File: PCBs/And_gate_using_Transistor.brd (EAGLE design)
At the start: 30 x 34.5 mm, 11 parts, among them T1 BC547, T2 BC547

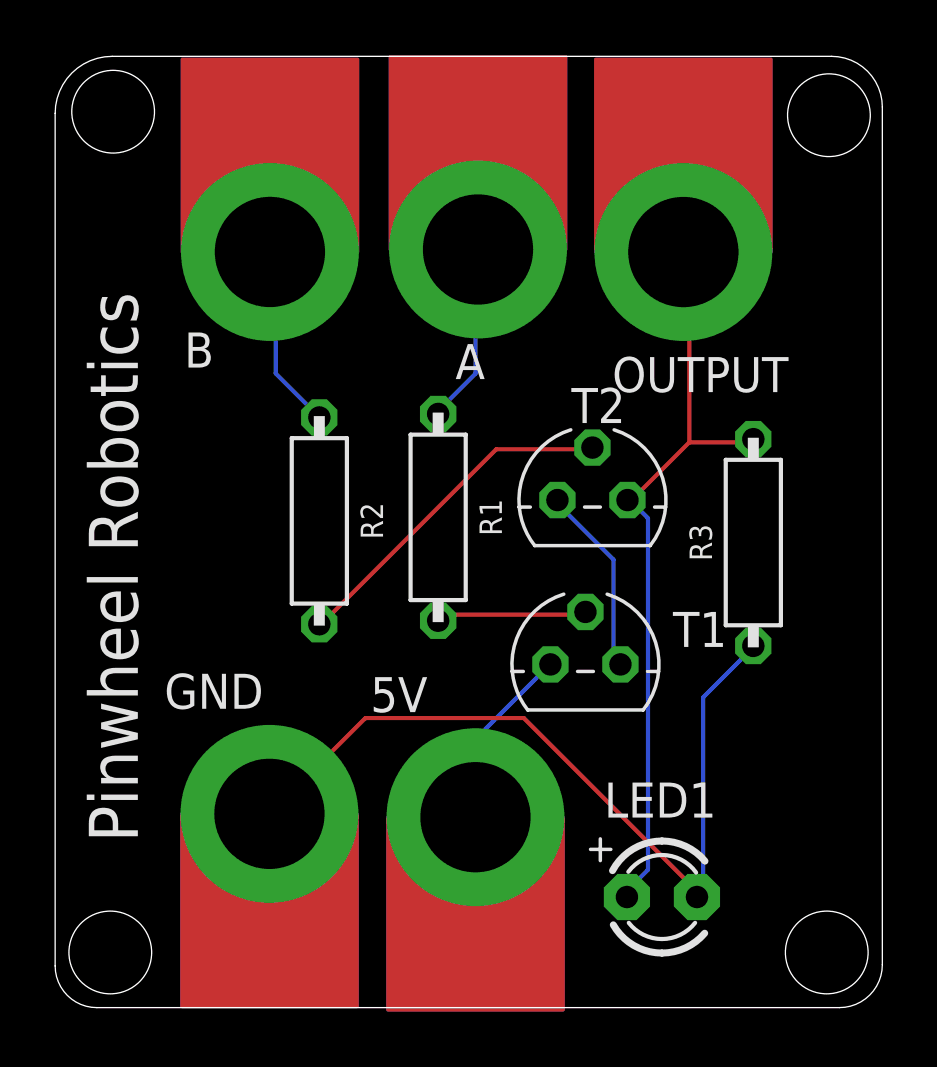
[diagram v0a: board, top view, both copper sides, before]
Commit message: New Update
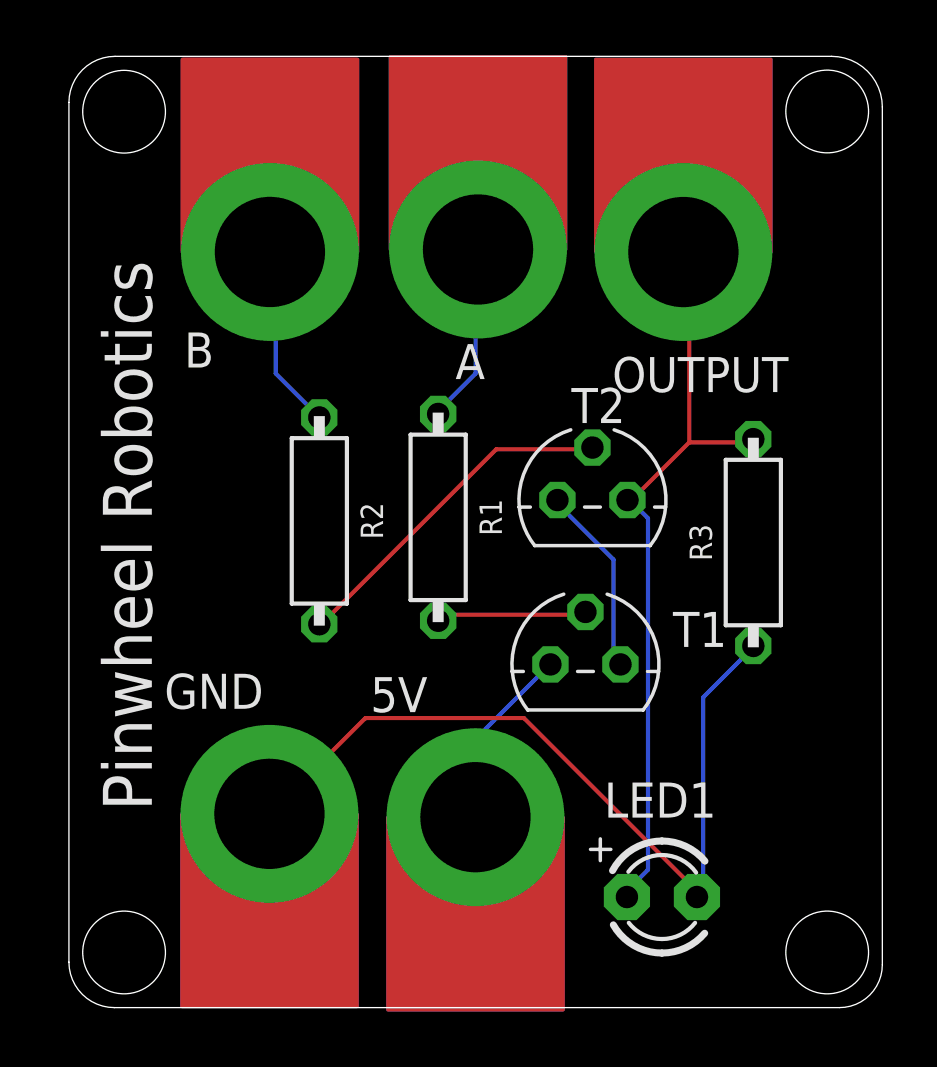
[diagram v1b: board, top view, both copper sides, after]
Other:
- board size 30 x 34.5 mm -> 29.5 x 34.5 mm
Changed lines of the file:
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@@
 <drawing>
 <settings>
-<setting alwaysvectorfont="yes"/>
+<setting alwaysvectorfont="no"/>
 <setting verticaltext="up"/>
 </settings>
@@
 <board>
 <plain>
-<wire x1="28.16231875" y1="34.5" x2="2.066921875" y2="34.5" width="0" layer="20"/>
-<wire x1="2.066921875" y1="34.5" x2="0" y2="32.433078125" width="0" layer="20" curve="90"/>
-<wire x1="0" y1="32.433078125" x2="0" y2="1.5111625" width="0" layer="20"/>
-<wire x1="0" y1="1.5111625" x2="1.5111625" y2="0" width="0" layer="20" curve="90"/>
-<wire x1="1.5111625" y1="0" x2="28.44391875" y2="0" width="0" layer="20"/>
+<wire x1="28.16231875" y1="34.5" x2="2.17199375" y2="34.5" width="0" layer="20"/>
+<wire x1="2.17199375" y1="34.5" x2="0.5" y2="32.82800625" width="0" layer="20" curve="90"/>
+<wire x1="0.5" y1="32.82800625" x2="0.5" y2="1.6494125" width="0" layer="20"/>
+<wire x1="0.5" y1="1.6494125" x2="2.1494125" y2="0" width="0" layer="20" curve="90"/>
+<wire x1="2.1494125" y1="0" x2="28.44391875" y2="0" width="0" layer="20"/>
 <wire x1="28.44391875" y1="0" x2="30" y2="1.55608125" width="0" layer="20" curve="90"/>
 <wire x1="30" y1="1.55608125" x2="30" y2="32.66231875" width="0" layer="20"/>
 <wire x1="30" y1="32.66231875" x2="28.16231875" y2="34.5" width="0" layer="20" curve="90"/>
-<hole x="2" y="2" drill="3"/>
-<hole x="27.984" y="2" drill="3"/>
-<hole x="28.063" y="32.365" drill="3"/>
-<hole x="2.103" y="32.492" drill="3"/>
-<text x="3" y="6" size="1.778" layer="21" rot="R90">Pinwheel Robotics </text>
+<hole x="2.5" y="2" drill="3"/>
+<hole x="28" y="2" drill="3"/>
+<hole x="28" y="32.5" drill="3"/>
+<hole x="2.5" y="32.492" drill="3"/>
+<text x="3.508" y="7.143" size="1.778" layer="21" rot="R90">Pinwheel Robotics </text>
 <text x="29.5" y="25" size="1.778" layer="22" rot="MR270">care@pinwheel</text>
 </plain>
